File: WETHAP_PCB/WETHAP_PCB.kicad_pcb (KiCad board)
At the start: 2 copper layers, 49 x 85 mm, 14 parts, among them J1 Conn_01x20_Socket, J2 Conn_01x20_Socket

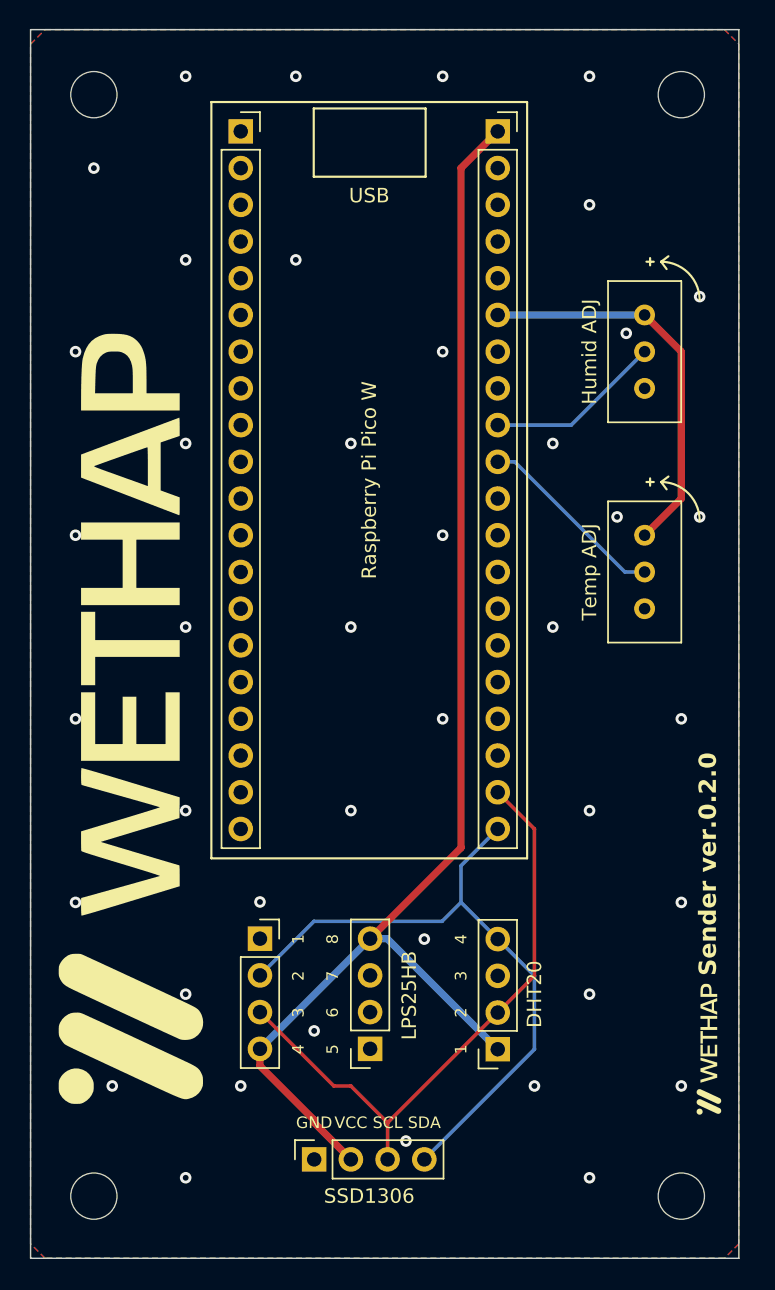
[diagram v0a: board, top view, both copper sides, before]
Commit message: fix circuit
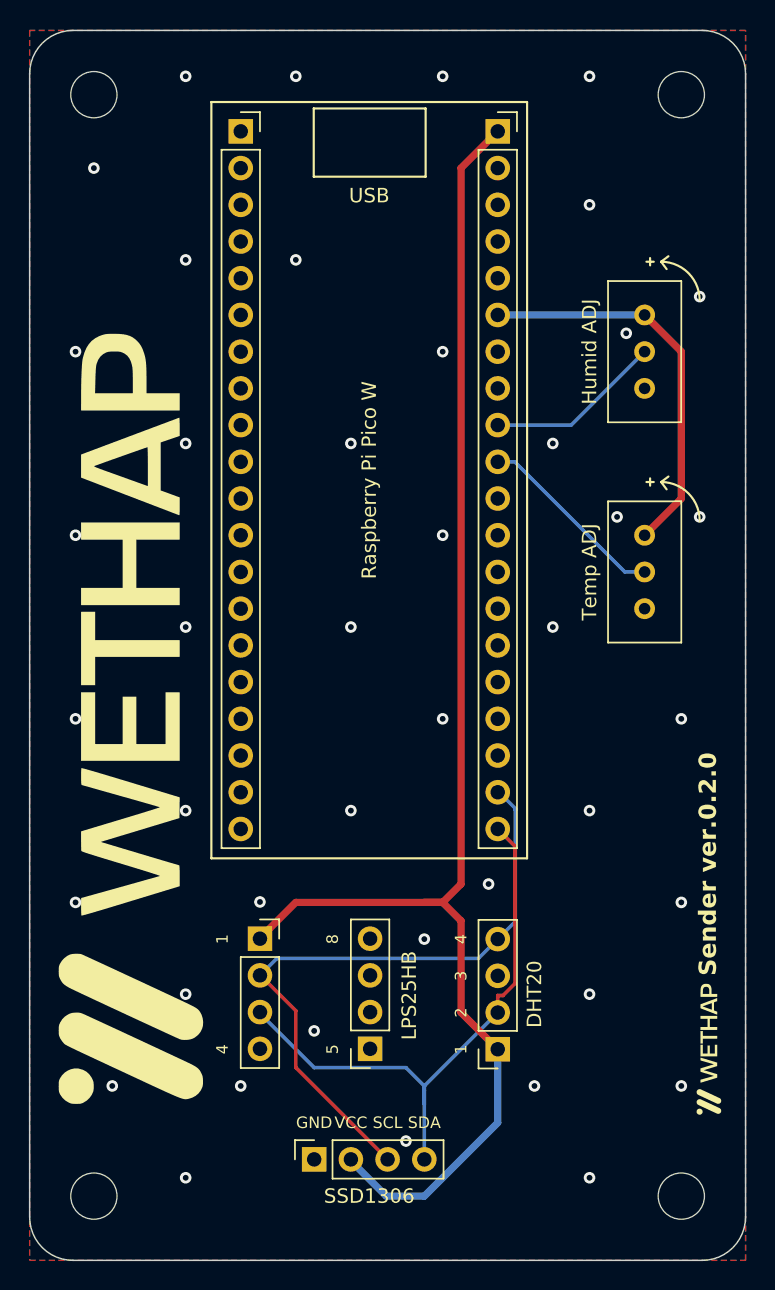
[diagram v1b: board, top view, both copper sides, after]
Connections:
- DHT20 pad 2: scl -> sda
- DHT20 pad 4: sda -> scl
- LPS25HB1 pad 1: gnd -> vbus
- LPS25HB1 pad 2: sda -> scl
- LPS25HB1 pad 3: scl -> sda
- LPS25HB1 pad 4: vbus -> gnd
- LPS25HB2 pad 1: gnd -> (no net)
- LPS25HB2 pad 2: unconnected-(LPS25HB2-Pin_2-Pad2) -> (no net)
- LPS25HB2 pad 3: unconnected-(LPS25HB2-Pin_3-Pad3) -> (no net)
- LPS25HB2 pad 4: vbus -> (no net)
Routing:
- net vbus: track 92.5 -> 100.1 mm
- net sda: track 45.2 -> 41.0 mm
- net scl: track 42.7 -> 45.2 mm
- net gnd: vias 42 -> 43
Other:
- board size 49 x 85 mm -> 49.5 x 85.1 mm
- board text removed: "6"
- board text removed: "7"
